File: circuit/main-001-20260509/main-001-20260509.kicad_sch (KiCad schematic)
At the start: 13 parts, among them Q3 BSS138, Q4 BSS138, U1 DEV-16771

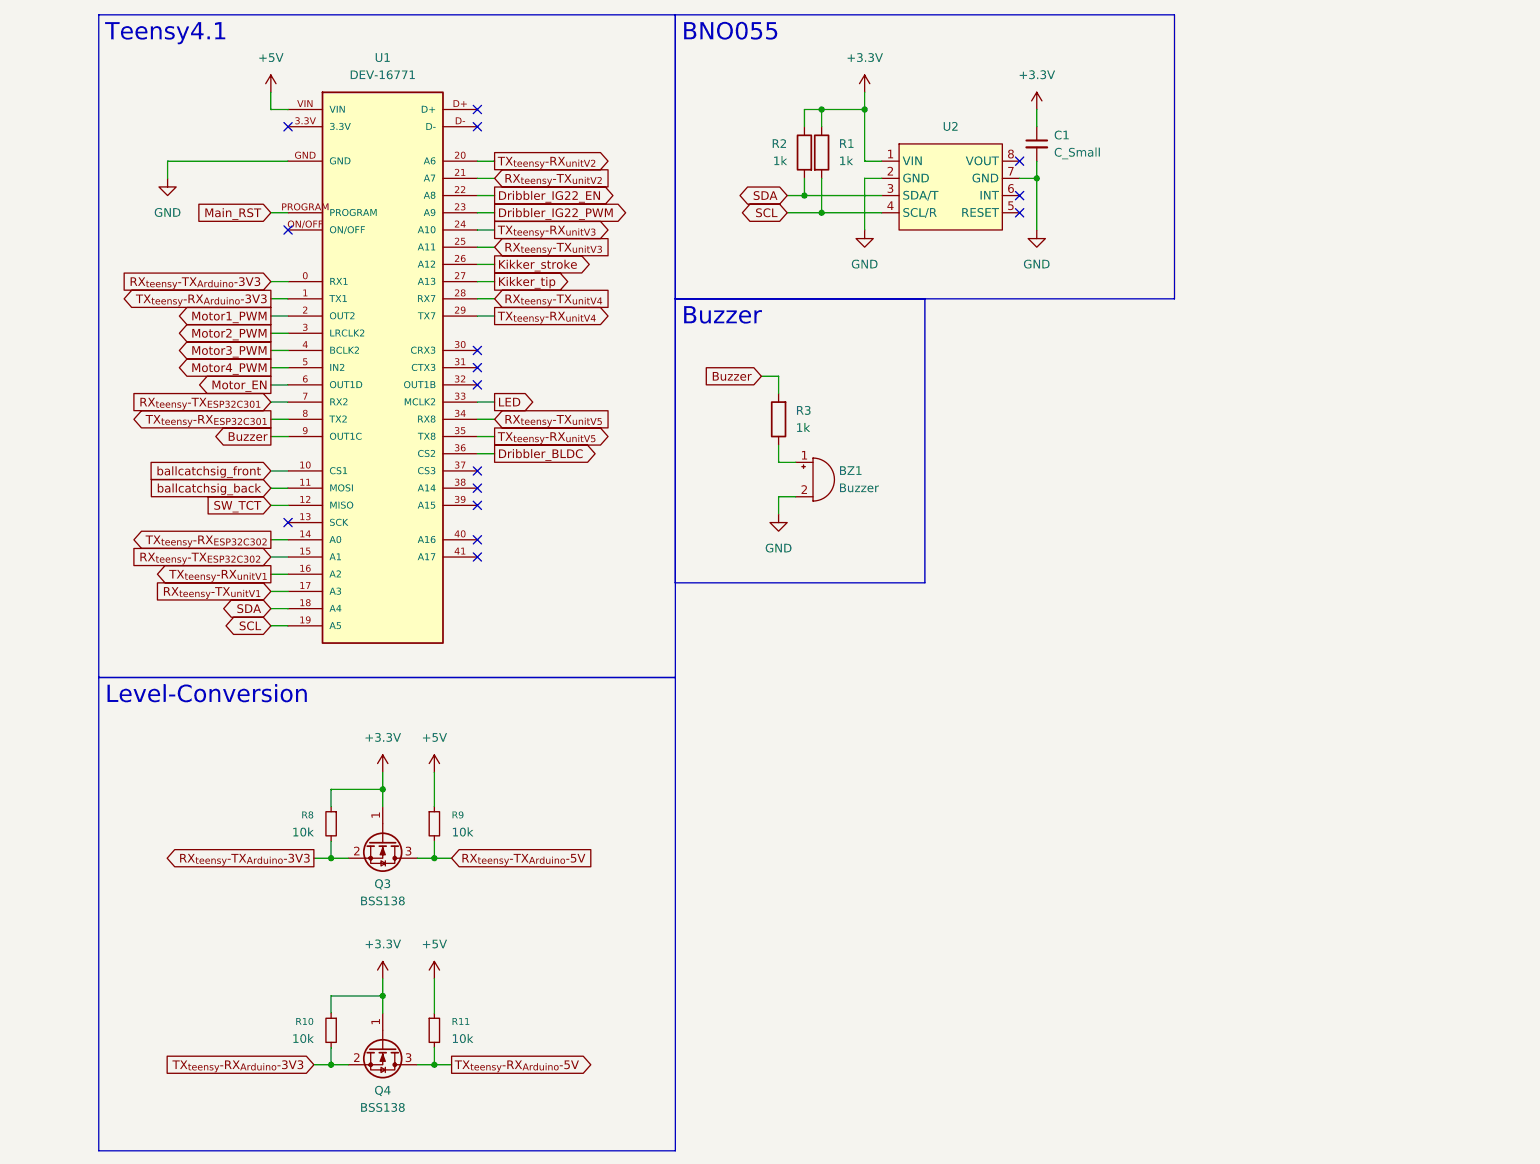
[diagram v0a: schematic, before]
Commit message: Update メイン基板の回路図仮完成
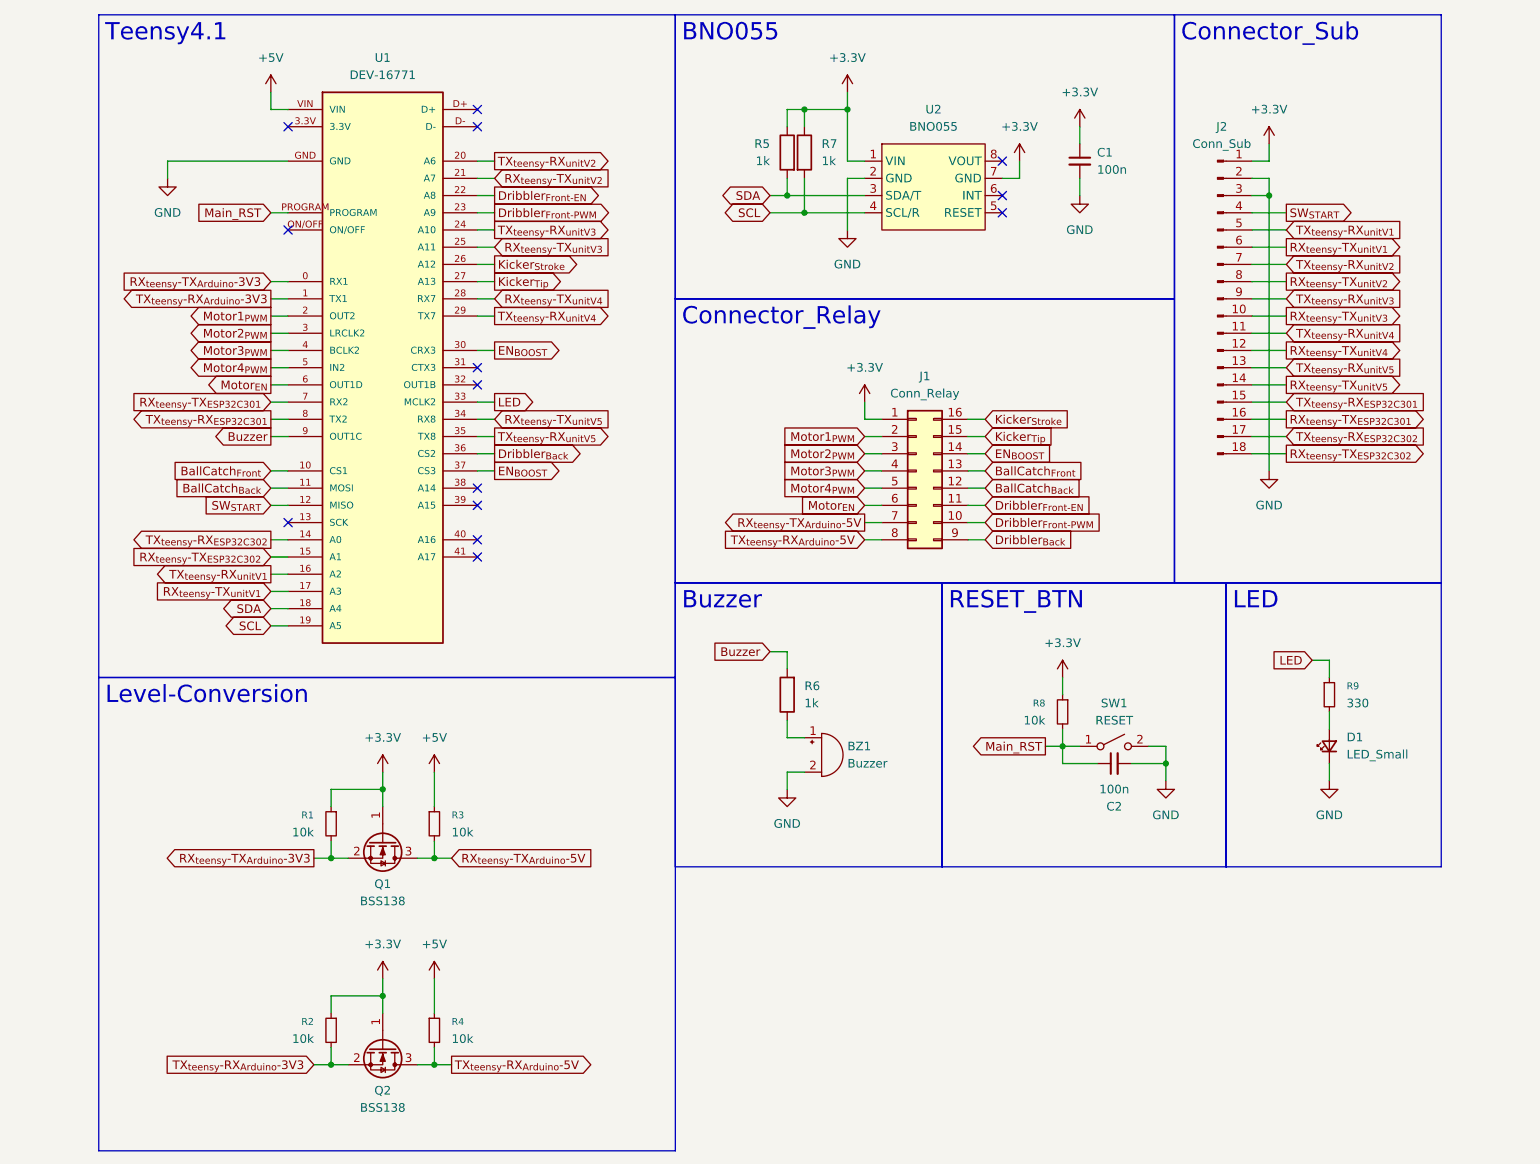
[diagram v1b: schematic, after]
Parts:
- added C2: 100n, Capacitor_SMD:C_0805_2012Metric, symbol Device:C_Small
- added D1: LED_Small, symbol Device:LED_Small
- added J1: Conn_Relay, Connector_PinSocket_2.54mm:PinSocket_2x08_P2.54mm_Vertical, symbol Connector_Generic:Conn_02x08_Counter_Clockwise
- added J2: Conn_Sub, symbol Connector:Conn_01x18_Pin
- added R8: 10k, Resistor_SMD:R_0805_2012Metric, symbol Device:R_Small
- added R9: 330, Resistor_SMD:R_0805_2012Metric, symbol Device:R_Small
- added SW1: RESET, symbol Switch:SW_SPST
- C1: value C_Small -> 100n; footprint (none) -> Capacitor_SMD:C_0805_2012Metric
- R1: renamed from R8; footprint (none) -> Resistor_SMD:R_0805_2012Metric
- R2: renamed from R10; footprint (none) -> Resistor_SMD:R_0805_2012Metric
- R3: renamed from R9; footprint (none) -> Resistor_SMD:R_0805_2012Metric
- R4: renamed from R11; footprint (none) -> Resistor_SMD:R_0805_2012Metric
- R5: renamed from R2; footprint (none) -> Resistor_SMD:R_0805_2012Metric
- R6: renamed from R3; footprint (none) -> Resistor_SMD:R_0805_2012Metric
- R7: renamed from R1; footprint (none) -> Resistor_SMD:R_0805_2012Metric
- U1: footprint @2024TOINIOT2-Main:MODULE_DEV-16771 -> @Thrive_footprint_main:DEV-16771
- U2: value (none) -> BNO055; footprint (none) -> @Thrive_footprint_main:BNO055
- renumbered Q3 to Q1, Q4 to Q2
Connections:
- net +3.3V: now also U2.7 (GND), J1.1 (Pin_1), J2.1 (Pin_1), R8.1
- net GND: now also C2.2, D1.1 (K), J2.2 (Pin_2), J2.3 (Pin_3), SW1.2 (B); no longer U2.7 (GND)
- net LED: now also R9.1
- net Main_RST: now also C2.1, R8.2, SW1.1 (A)
- net RX_{teensy}-TX_{Arduino}-5V: now also J1.7 (Pin_7)
- net RX_{teensy}-TX_{ESP32C301}: now also J2.16 (Pin_16)
- net RX_{teensy}-TX_{ESP32C302}: now also J2.18 (Pin_18)
- net RX_{teensy}-TX_{unitV1}: now also J2.6 (Pin_6)
- net RX_{teensy}-TX_{unitV2}: now also J2.8 (Pin_8)
- net RX_{teensy}-TX_{unitV3}: now also J2.10 (Pin_10)
- net RX_{teensy}-TX_{unitV4}: now also J2.12 (Pin_12)
- net RX_{teensy}-TX_{unitV5}: now also J2.14 (Pin_14)
- net TX_{teensy}-RX_{Arduino}-5V: now also J1.8 (Pin_8)
- net TX_{teensy}-RX_{ESP32C301}: now also J2.15 (Pin_15)
- net TX_{teensy}-RX_{ESP32C302}: now also J2.17 (Pin_17)
- net TX_{teensy}-RX_{unitV1}: now also J2.5 (Pin_5)
- net TX_{teensy}-RX_{unitV2}: now also J2.7 (Pin_7)
- net TX_{teensy}-RX_{unitV3}: now also J2.9 (Pin_9)
- net TX_{teensy}-RX_{unitV4}: now also J2.11 (Pin_11)
- net TX_{teensy}-RX_{unitV5}: now also J2.13 (Pin_13)
- net EN_{BOOST}: now reaches U1.30 (CRX3)
- net EN_{BOOST}: now also U1.37 (CS3), J1.14 (Pin_14)
- net Dribbler_BLDC renamed Dribbler_{Back}
- net Dribbler_{Back}: now also J1.9 (Pin_9)
- net Dribbler_IG22_EN renamed Dribbler_{Front-EN}
- net Dribbler_{Front-EN}: now also J1.11 (Pin_11)
- net Dribbler_IG22_PWM renamed Dribbler_{Front-PWM}
- net Dribbler_{Front-PWM}: now also J1.10 (Pin_10)
- net Kikker_stroke renamed Kicker_{Stroke}
- net Kicker_{Stroke}: now also J1.16 (Pin_16)
- net Kikker_tip renamed Kicker_{Tip}
- net Kicker_{Tip}: now also J1.15 (Pin_15)
- net Motor1_PWM renamed Motor1_{PWM}
- net Motor1_{PWM}: now also J1.2 (Pin_2)
- net Motor2_PWM renamed Motor2_{PWM}
- net Motor2_{PWM}: now also J1.3 (Pin_3)
- net Motor3_PWM renamed Motor3_{PWM}
- net Motor3_{PWM}: now also J1.4 (Pin_4)
- net Motor4_PWM renamed Motor4_{PWM}
- net Motor4_{PWM}: now also J1.5 (Pin_5)
- net Motor_EN renamed Motor_{EN}
- net Motor_{EN}: now also J1.6 (Pin_6)
- net SW_TCT renamed SW_{START}
- net SW_{START}: now also J2.4 (Pin_4)
- net ballcatchsig_back renamed BallCatch_{Back}
- net BallCatch_{Back}: now also J1.12 (Pin_12)
- net ballcatchsig_front renamed BallCatch_{Front}
- net BallCatch_{Front}: now also J1.13 (Pin_13)
- new net: D1.2 (A), R9.2
- no-connect marks 16 -> 14
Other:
- moved on the sheet: BZ1, C1, R5, R6, R7
